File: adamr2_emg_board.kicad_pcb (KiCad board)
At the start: 2 copper layers, 60 x 45 mm, 6 parts, among them J1 Screw_Terminal_01x04, J2 Conn_01x02, K1 G6C-1114P-US

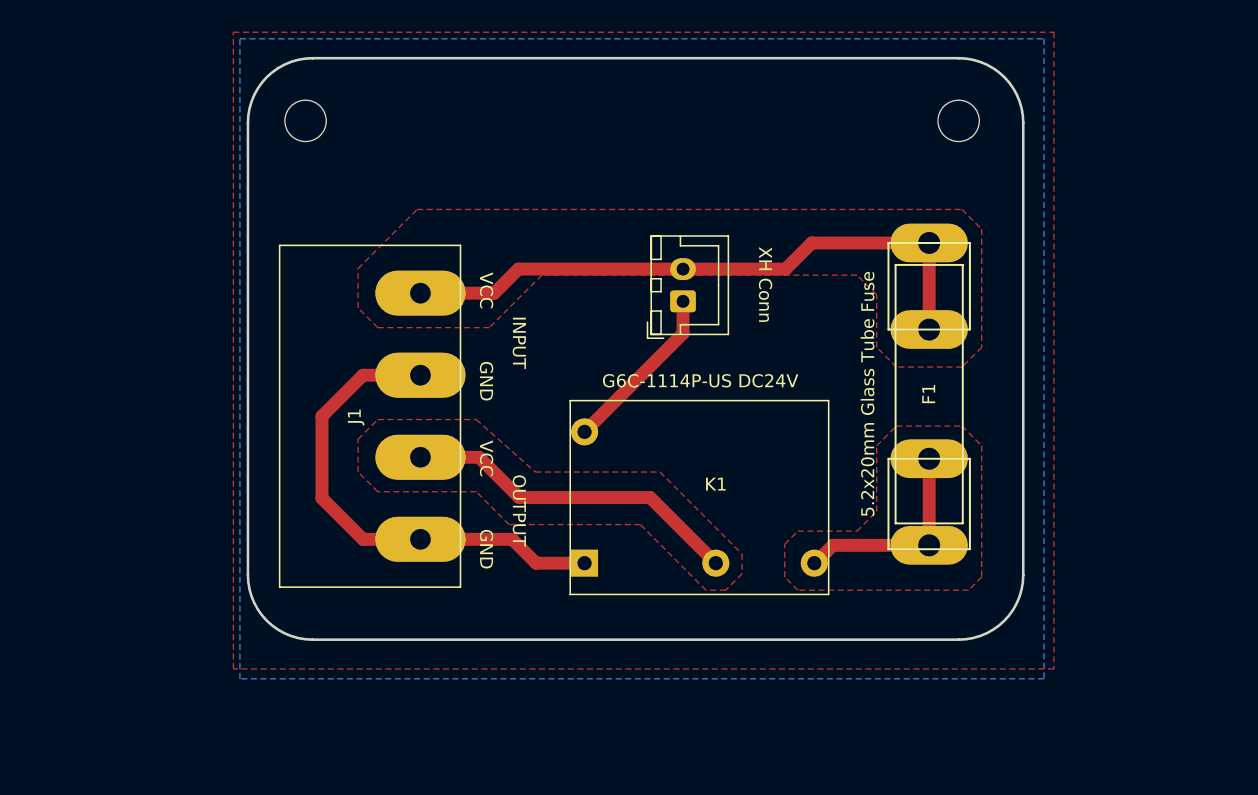
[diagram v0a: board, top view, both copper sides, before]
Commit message: Update
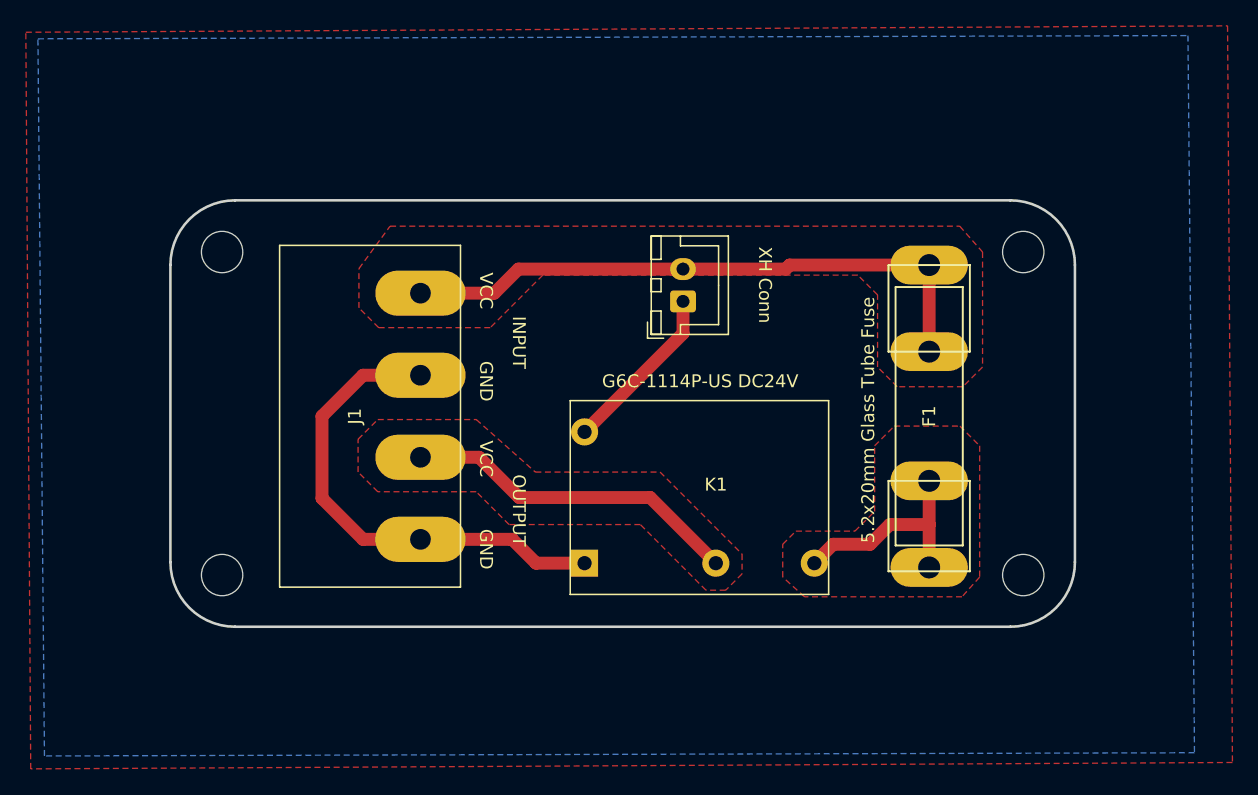
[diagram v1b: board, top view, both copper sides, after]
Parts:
- added REF**: MountingHole_3.2mm_M3, MountingHole:MountingHole_3.2mm_M3, F.Cu at (118.0, 105.0)
- added REF**: MountingHole_3.2mm_M3, MountingHole:MountingHole_3.2mm_M3, F.Cu at (180.0, 105.0)
- moved REF** 12.0 mm to (118.0, 80.0)
- moved REF** 11.3 mm to (180.0, 80.0)
- moved F1 1.71 mm to (172.7, 92.7)
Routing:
- net VCC: track 48.4 -> 47.0 mm
- net Net-(F1-Pad2): track 16.2 -> 16.9 mm
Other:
- board size 60 x 45 mm -> 70 x 33 mm
